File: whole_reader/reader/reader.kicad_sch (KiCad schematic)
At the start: 67 parts, among them U1 LM386M-1, U2 STM32F103C8T6, U3 MCP16301Hx-xCH, U4 TP3232N-SR, Y1 16MHz

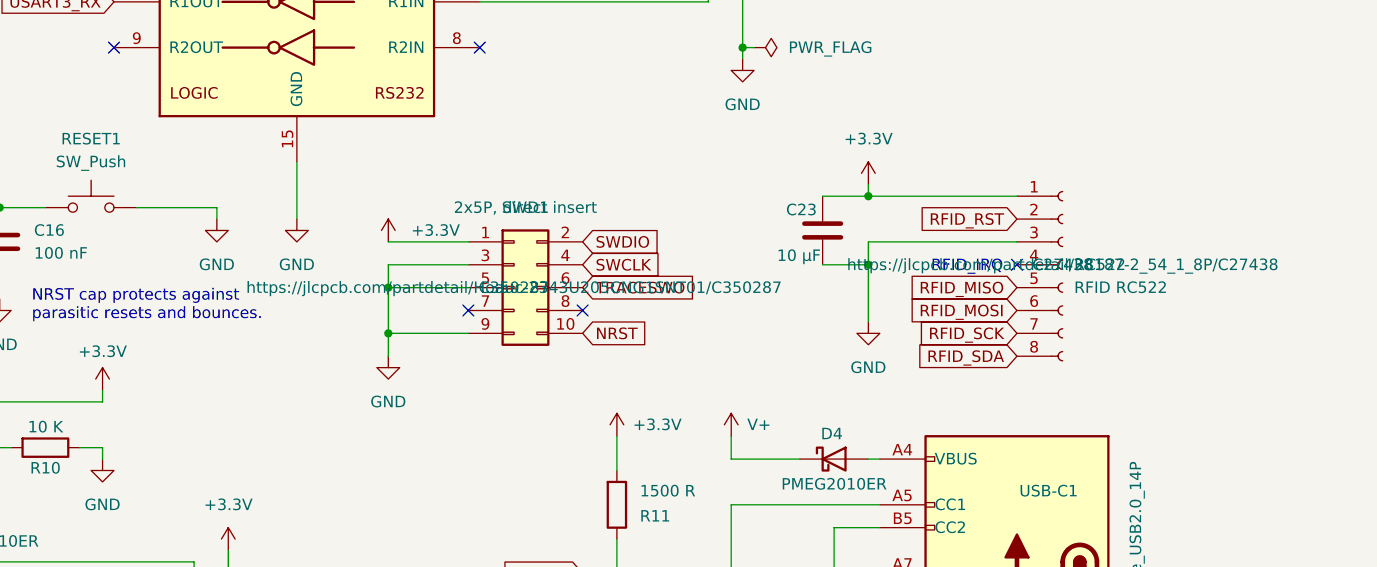
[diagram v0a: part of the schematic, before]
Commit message: updates on pcb, bom file and experimenting with footprints
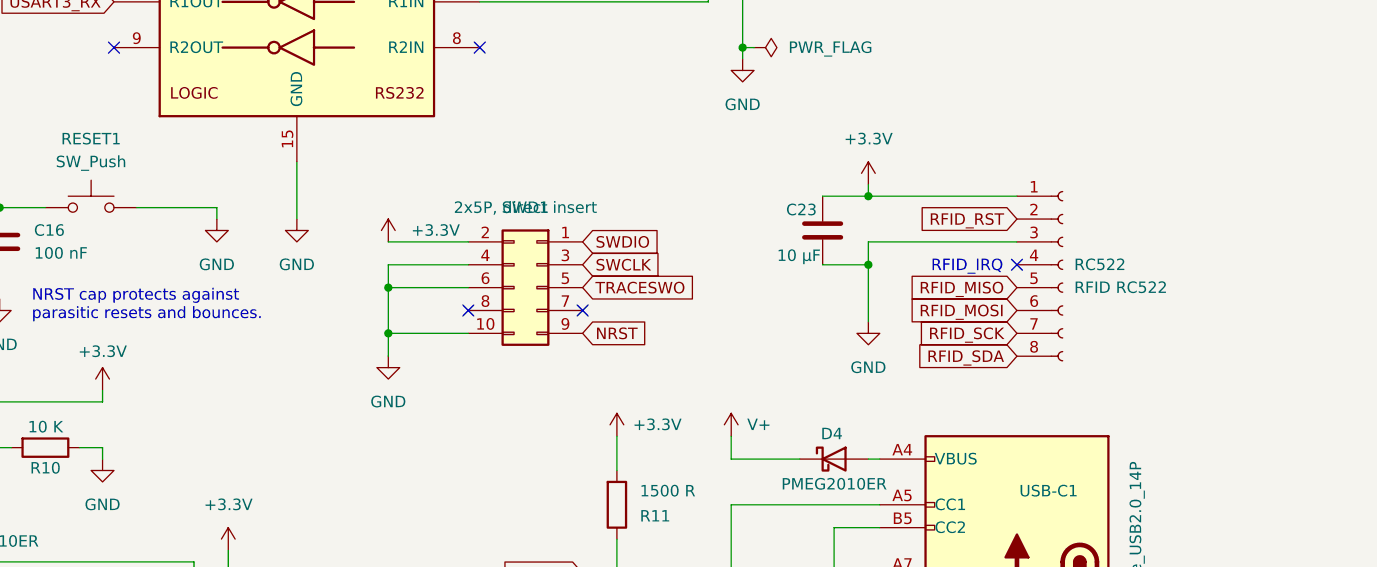
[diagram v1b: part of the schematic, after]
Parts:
- BOOT1: JLCPCB https://jlcpcb.com/partdetail/ck-PCM12SMTR/C221841 -> https://jlcpcb.com/partdetail/Alpsalpine-SSSS811101/C109335; LCSC C221841 -> C109335
- L1: JLCPCB https://jlcpcb.com/partdetail/Coilcraft-LPS3010103MRC/C1927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 -> https://jlcpcb.com/partdetail/Ceaiya-CR3012150M/C520285; LCSC C19276043 -> C520285
- LED2: JLCPCB https://jlcpcb.com/partdetail/Kingbright-APHBM2012LSURKZGKC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 -> https://jlcpcb.com/partdetail/Kingbright-APHBM2012SURKCGKC/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; LCSC C6465979 -> C5553822
- R1: JLCPCB https://jlcpcb.com/partdetail/Sunway-SC0805J1003F4ANRH/C315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 -> https://jlcpcb.com/partdetail/160838-0805W8F1003T5E/C149504; LCSC C3152215 -> C149504
- R2: footprint Potentiometer_SMD:Potentiometer_Bourns_3314S_Horizontal -> Potentiometer_SMD:Potentiometer_Bourns_3314G_Vertical
- R3: JLCPCB https://jlcpcb.com/partdetail/25882-0402WGJ0100TCE/C25139 -> https://jlcpcb.com/partdetail/25820-0402WGF100JTCE/C25077; LCSC C25139 -> C25077
- RC522: footprint Connector_PinSocket_2.54mm:PinSocket_1x08_P2.54mm_Vertical -> UACS:PinSocket_1x08_P2.54mm_Vertical
- SWD1: footprint Connector_PinSocket_1.27mm:PinSocket_2x05_P1.27mm_Vertical -> UACS:PinSocket_2x05_P1.27mm_Vertical
- USB-C1: JLCPCB https://jlcpcb.com/partdetail/5762033-USB4110_GFA/C5143397 -> https://jlcpcb.com/partdetail/ShouHan-TYPE_C_16PIN_2MD_073/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; LCSC C5143397 -> C2765186
- Y1: JLCPCB https://jlcpcb.com/partdetail/Yajingxin-TX322516M4DBDE2T/C5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 -> https://jlcpcb.com/partdetail/Yxc_CrystalOscillators-X32251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; LCSC C5310731 -> C13738
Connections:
- net +3.3V: now also SWD1.2 (Pin_2); no longer SWD1.1 (Pin_1)
- net GND: now also SWD1.10 (Pin_10), SWD1.4 (Pin_4), SWD1.6 (Pin_6); no longer SWD1.3 (Pin_3), SWD1.5 (Pin_5), SWD1.9 (Pin_9)
- net NRST: now also SWD1.9 (Pin_9); no longer SWD1.10 (Pin_10)
- net SWCLK: now also SWD1.3 (Pin_3); no longer SWD1.4 (Pin_4)
- net SWDIO: now also SWD1.1 (Pin_1); no longer SWD1.2 (Pin_2)
- net TRACESWO: now also SWD1.5 (Pin_5); no longer SWD1.6 (Pin_6)

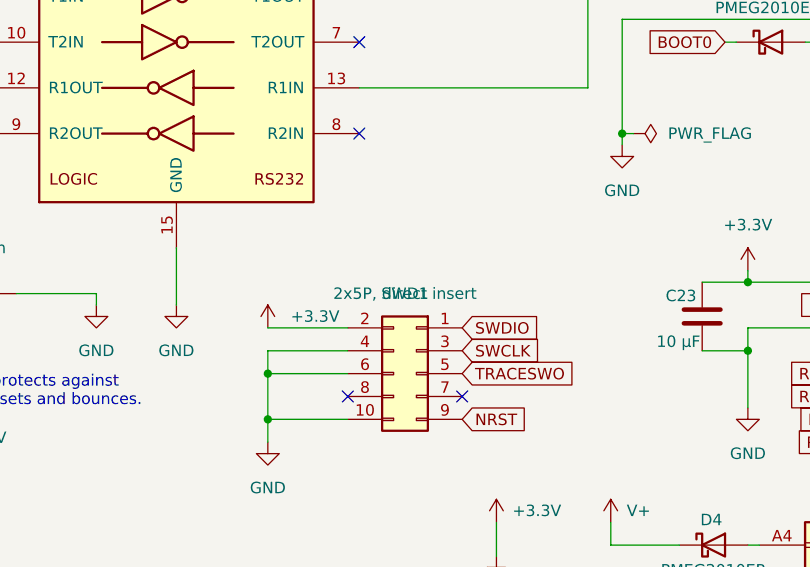
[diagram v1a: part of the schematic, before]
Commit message: Úprava popisov
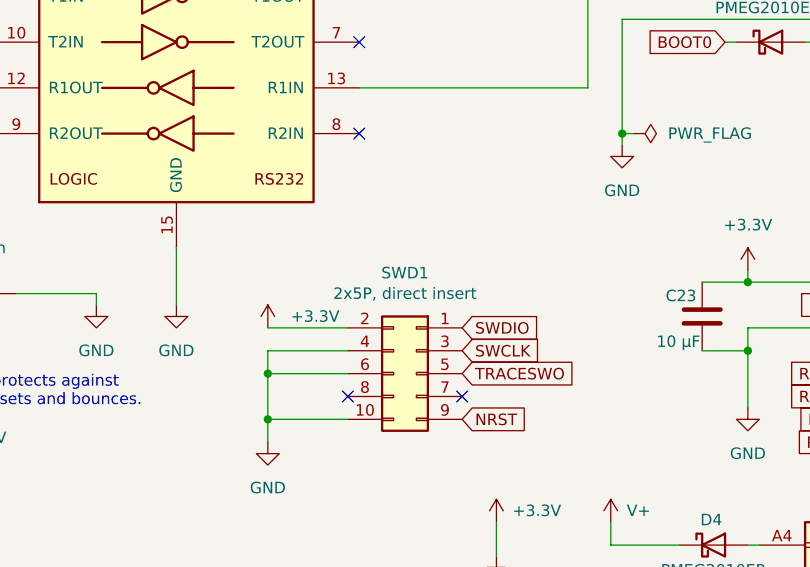
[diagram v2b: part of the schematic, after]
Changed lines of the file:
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@@
 			"MDk0MykoeHkgMy40ODI5MjUgLTMuNTA3NzYxKSh4eSAzLjEzODk2OCAtMi45NTQ1NzgpKHh5IDIu"
 			"OTU3NjY3IC0yLjk0OTIwOSkoeHkgMi43NzYzNjUgLTIuOTQzODQpKHh5IDIuNzc2MzY1IC0zLjc2"
-			"OTkyNikoeHkgLTEuMTQyMjY1IC0zLjc2OQ=="
+			"OTkyNikoeHkgLTEuMTQyMjY1IC0zLjc2OQAAAAAAAAAAAAAAAAAAAAAAAAAAAAAAAAAAAAAAAAAA"
+			"AAAAAAAAAAAAAAAAAAAAAAAAAAAAAAAAAAAAAAAAAAAAAAAAAAAAAAAAAAAAAAAAAAAAAAAAAAAA"
+			"AAAAAAAAAAAAAAAAAAAAAAAAAAAAAAAAAAAAAAAAAAAAAAAAAAAAAAAAAAAAAAAAAAAAAAAAAAAA"
+			"AAAAAAAAAAAAAAAAAAAAAAAAAAAAAAAAAAAAAAAAAAAAAAAAAAAAAAAAAAAAAAAAAAAAAAAAAAAA"
+			"AAAAAAAAAAAAAAAAAAAAAAAAAAAAAAAAAAAAAAAAAAAAAAAAAAAAAAAAAAAAAAAAAAAAAAAAAAAA"
+			"AAAAAAAAAAAAAAAAAAAAAAAAAAAAAAAAAAAAAAAAAAAAAAAAAAAAAAAAAAAAAAAAAAAAAAAAAAAA"
+			"AAAAAAAAAAAAAAAAAAAAAAAAAAAAAAAAAAAAAAAAAAAAAAAAAAAAAAAAAAAAAAAAAAAAAAAAAAAA"
+			"AAAAAAAAAAAAAAAAAAAAAAAAAAAAAAAAAAAAAAAAAAAAAAAAAAAAAAAAAAAAAAAAAAAAAAAAAAAA"
+			"AAAAAAAAAAAAAAAAAAAAAAAAAAAAAAAAAAAAAAAAAAAAAAAAAAAAAAAAAAAAAAAAAAAAAAAAAAAA"
+			"AAAAAAAAAAAAAAAAAAAAAAAAAAAAAAAAAAAAAAAAAAAAAAAAAAAAAAAAAAAAAAAAAAAAAAAAAAAA"
+			"AAAAAAAAAAAAAAAAAAAAAAAAAAAAAAAAAAAAAAAAAAAAAAAAAAAAAAAAAAAAAAAAAAAAAAAAAAAA"
+			"AAAAAAAAAAAAAAAAAAAAAAAAAAAAAAAAAAAAAAAAAAAAAAAAAAAAAAAAAAAAAAAAAAAAAAAAAAAA"
+			"AAAAAAAAAAAAAAAAAAAAAAAAAAAAAAAAAAAAAAAAAAAAAAAAAAAAAAAAAAAAAAAAAAAAAAAAAAAA"
+			"AAAAAAAAAAAAAAAAAAAAAAAAAAAAAAAAAAAAAAAAAAAAAAAAAAAAAAAAAAAAAAAAAAAAAAAAAAAA"
+			"AAAAAAAAAAAAAAAAAAAAAAAAAAAAAAAAAAAAAAAAAAAAAAAAAAAAAAAAAAAAAAAAAAAAAAAAAAAA"
+			"AAAAAAAAAAAAAAAAAAAAAAAAAAAAAAAAAAAAAAAAAAAAAAAAAAAAAAAAAAAAAAAAAAAAAAAAAAAA"
+			"AAAAAAAAAAAAAAAAAAAAAAAAAAAAAAAAAAAAAAAAAAAAAAAAAAAAAAAAAAAAAAAAAAAAAAAAAAAA"
+			"AAAAAAAAAAAAAAAAAAAAAAAAAAAAAAAAAAAAAAAAAAAAAAAAAAAAAAAAAAAAAAAAAAAAAAAAAAAA"
+			"AAAAAAAAAAAAAAAAAAAAAAAAAAAAAAAAAA=="
 		)
 	)
@@
 			"cwBXAEsANwBoAEIAOABwAGcAUAAwAHYAagB1AGgAYQBQADIAMAB2AFQAcwBoAEEAegBkAHAAaQBq"
 			"AHUAaABDAEgAMgAxAGkAagB1AGgAdwBqAGkARgAyAEwAZwBsADMAUQBGAEEAWgB6AEIAQwBSAEwA"
-			"awArADUAdwA0AG8Adw=="
+			"awArADUAdwA0AG8AdwAAAAAAAAAAAAAAAAAAAAAAAAAAAAAAAAAAAAAAAAAAAAAAAAAAAAAAAAAA"
+			"AAAAAAAAAAAAAAAAAAAAAAAAAAAAAAAAAAAAAAAAAAAAAAAAAAAAAAAAAAAAAAAAAAAAAAAAAAAA"
+			"AAAAAAAAAAAAAAAAAAAAAAAAAAAAAAAAAAAAAAAAAAAAAAAAAAAAAAAAAAAAAAAAAAAAAAAAAAAA"
+			"AAAAAAAAAAAAAAAAAAAAAAAAAAAAAAAAAAAAAAAAAAAAAAAAAAAAAAAAAAAAAAAAAAAAAAAAAAAA"
+			"AAAAAAAAAAAAAAAAAAAAAAAAAAAAAAAAAAAAAAAAAAAAAAAAAAAAAAAAAAAAAAAAAAAAAAAAAAAA"
+			"AAAAAAAAAAAAAAAAAAAAAAAAAAAAAAAAAAAAAAAAAAAAAAAAAAAAAAAAAAAAAAAAAAAAAAACAAAA"
+			"AAAAAAAAAAAAAAAAAAAAAAAAAAAAAAAAAAAAAAAAAAAAAAAAAAAAAAAAAAAAAAAAAAAAAAAAAAAA"
+			"AAAAAAAAAAAAAAAAAAAAAAAAAAAAAAAAAAAAAAAAAAAAAAAAAAAAAAAAAAAAAAAAAAAAAAAAAAAA"
+			"AAAAAAAAAAAAAAAAAAAAAAAAAAAAAAAAAAAAAAAAAAAAAAAAAAAAAAAAAAAAAAAAAAAAAAAAAAAA"
+			"AAAAAAAAAAAAAAAAAAAAAAAAAAAAAAAAAAAAAAAAAAAAAAAAAAAAAAAAAAAAAAAAAAAAAAAAAAAA"
+			"AAAAAAAAAAAAAAAAAAAAAAAAAAAAAAAAAAAAAAAAAAAAAAAAAAAAAAAAAAAAAAAAAAAAAAAAAAAA"
+			"AAAAAAAAAAAAAAAAAAAAAAAAAAAAAAAAAAAAAAAAAAAAAAAAAAAAAAAAAAAAAAAAAAAAAAAAAAAA"
+			"AAAAAAAAAAAAAAAAAAAAAAAAAAAAAAAAAAAAAAAAAAAAAAAAAAAAAAAAAAAAAAAAAAAAAAAAAAAA"
+			"AAAAAAAAAAAAAAAAAAAAAAAAAAAAAAAAAAAAAAAAAAAAAAAAAAAAAAAAAAAAAAAAAAAAAAAAAAAA"
+			"AAAAAAAAAAAAAAAAAAAAAAAAAAAAAAAAAAAAAAAAAAAAAAAAAAAAAAAAAAAAAAAAAAAAAAAAAAAA"
+			"AAAAAAAAAAAAAAAAAAAAAAAAAAAAAAAAAAAAAAAAAAAAAAAAAAAAAAAAAAAAAAAAAAAAAAAAAAAA"
+			"AAAAAAAAAAAAAAAAAAAAAAAAAAAAAAAAAAAAAAAAAAAAAAAAAAAAAAAAAAAAAAAAAAAAAAAAAAAA"
+			"AAAAAAAAAAAAAAAAAAAAAAAAAAAAAAAAAAAAAAAAAAAAAAAAAAAAAAAAAAAAAAAAAAAAAAAAAAAA"
+			"AAAAAAAAAAAAAAAAAA=="
 		)
 	)
@@
 		(dnp no)
 		(property "Reference" "SWD1"
-			(at 209.55 92.71 0)
+			(at 209.55 90.424 0)
 			(effects
 				(font
